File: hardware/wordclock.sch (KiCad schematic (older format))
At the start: 15 parts, among them K1 SERIAL, P1 ISP, P2 Vin, U1 ATmega168, U2 DS1307, U3 7805, U4 4094, U5 4017, X1 32.768kHz

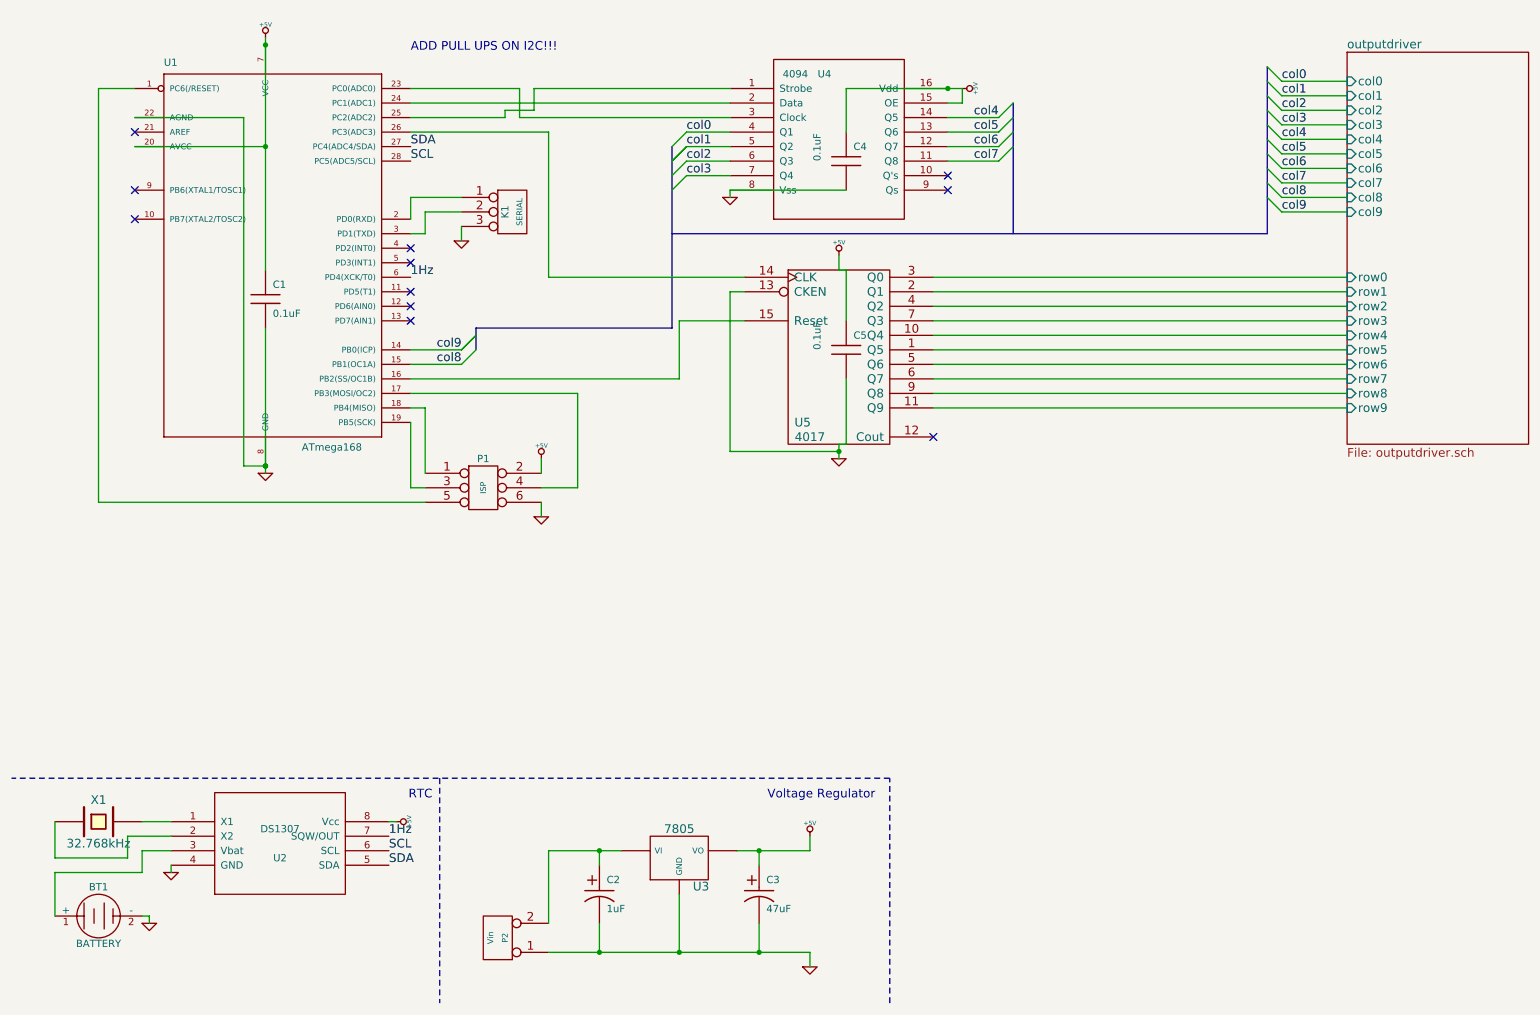
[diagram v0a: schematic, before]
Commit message: REV. A PCB nearly complete.
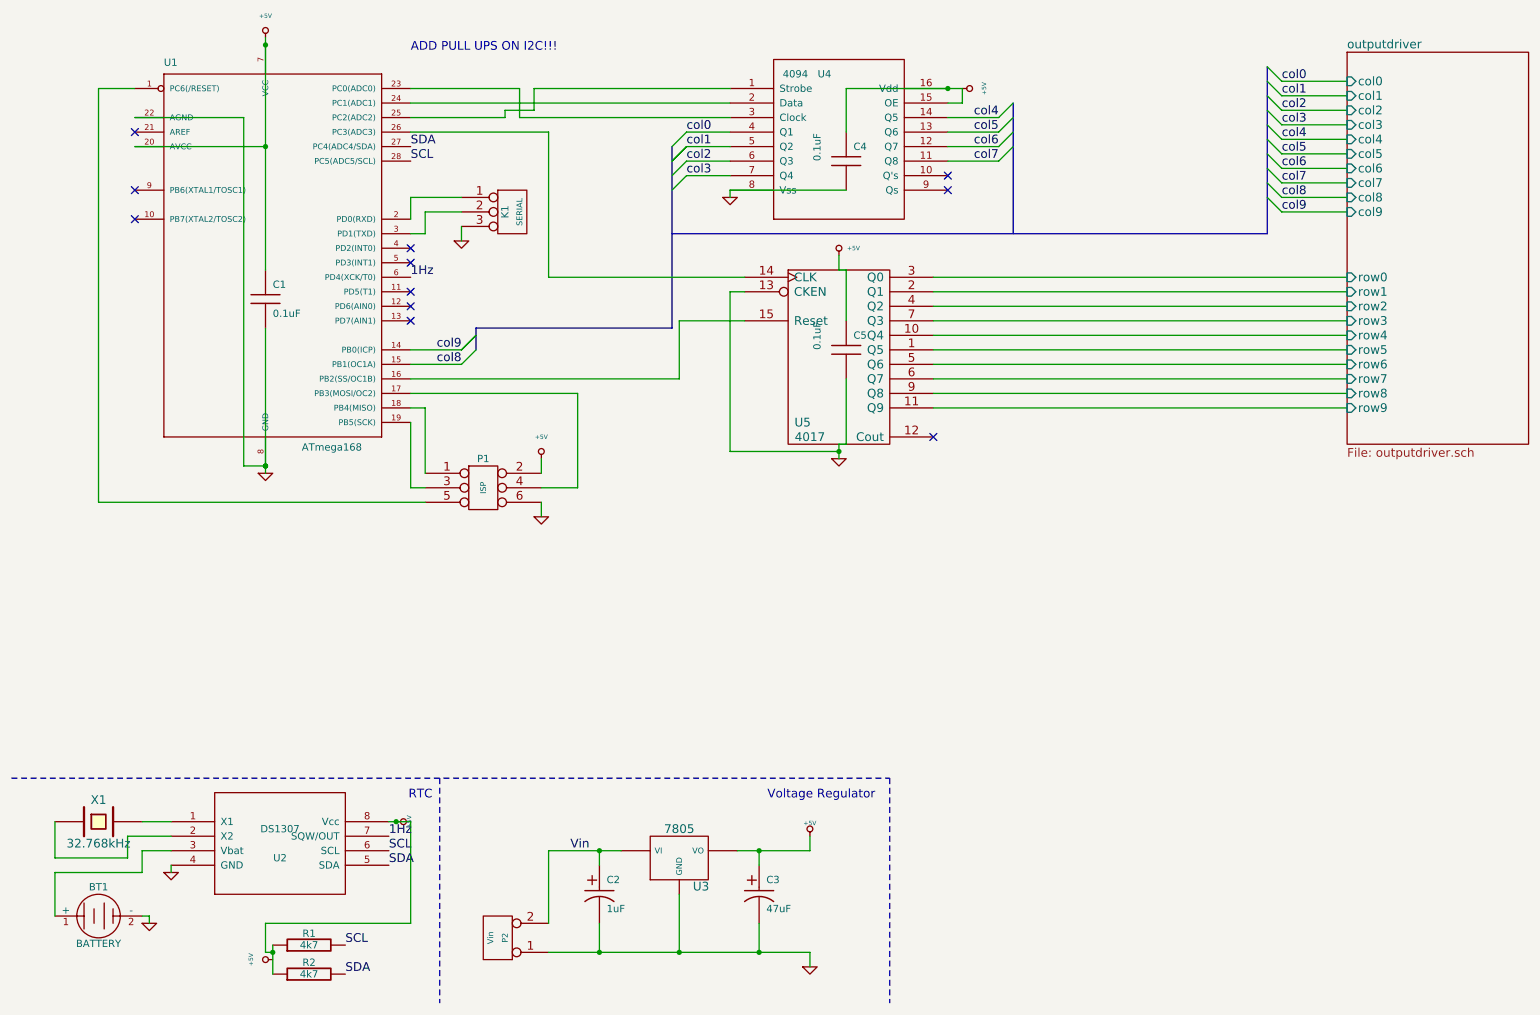
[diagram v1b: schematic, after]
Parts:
- added R1, R2: 4k7, symbol R
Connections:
- net +5V: now also R1.1, R2.1
- net SCL: now also R1.2
- net SDA: now also R2.2
- net Vin: now reaches C2.1, P2.2 (PM), U3.1 (VI)
